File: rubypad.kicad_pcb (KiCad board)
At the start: 2 copper layers, 13 parts, among them U1 ProMicro

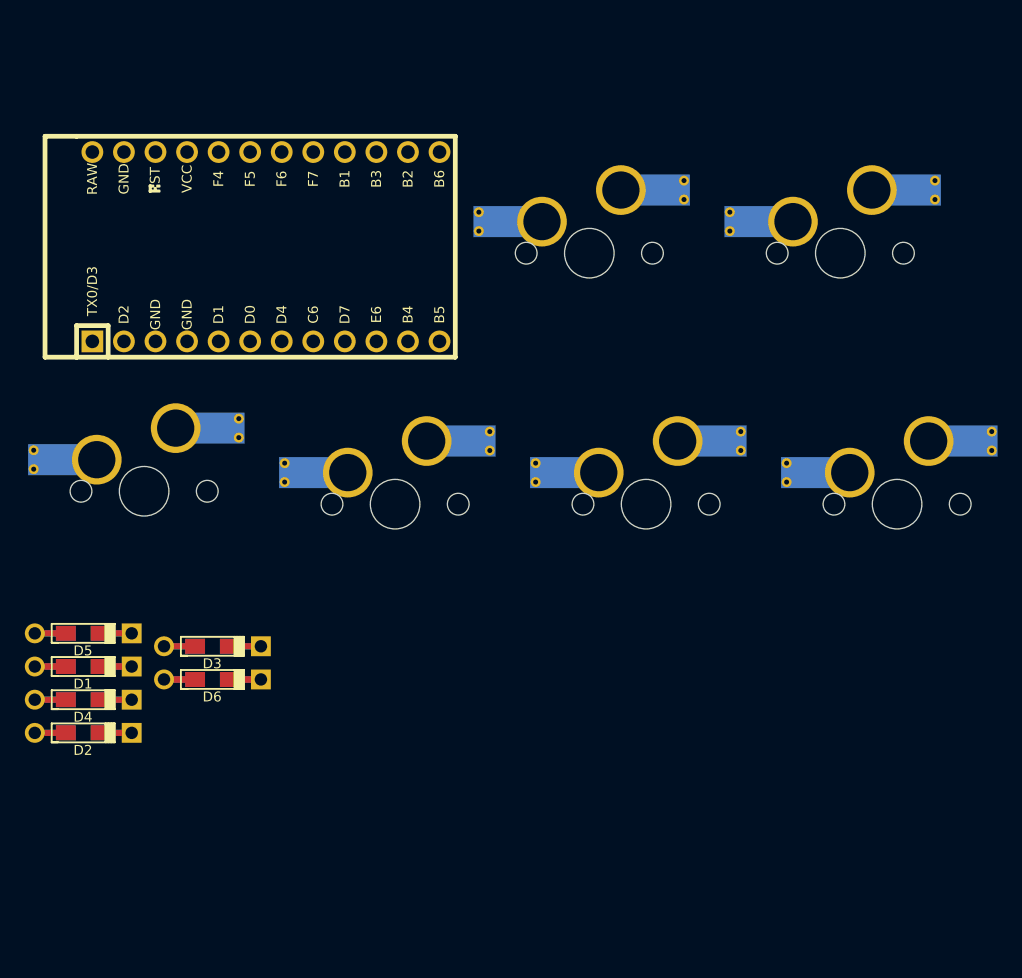
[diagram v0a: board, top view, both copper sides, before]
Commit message: Update - ran traces
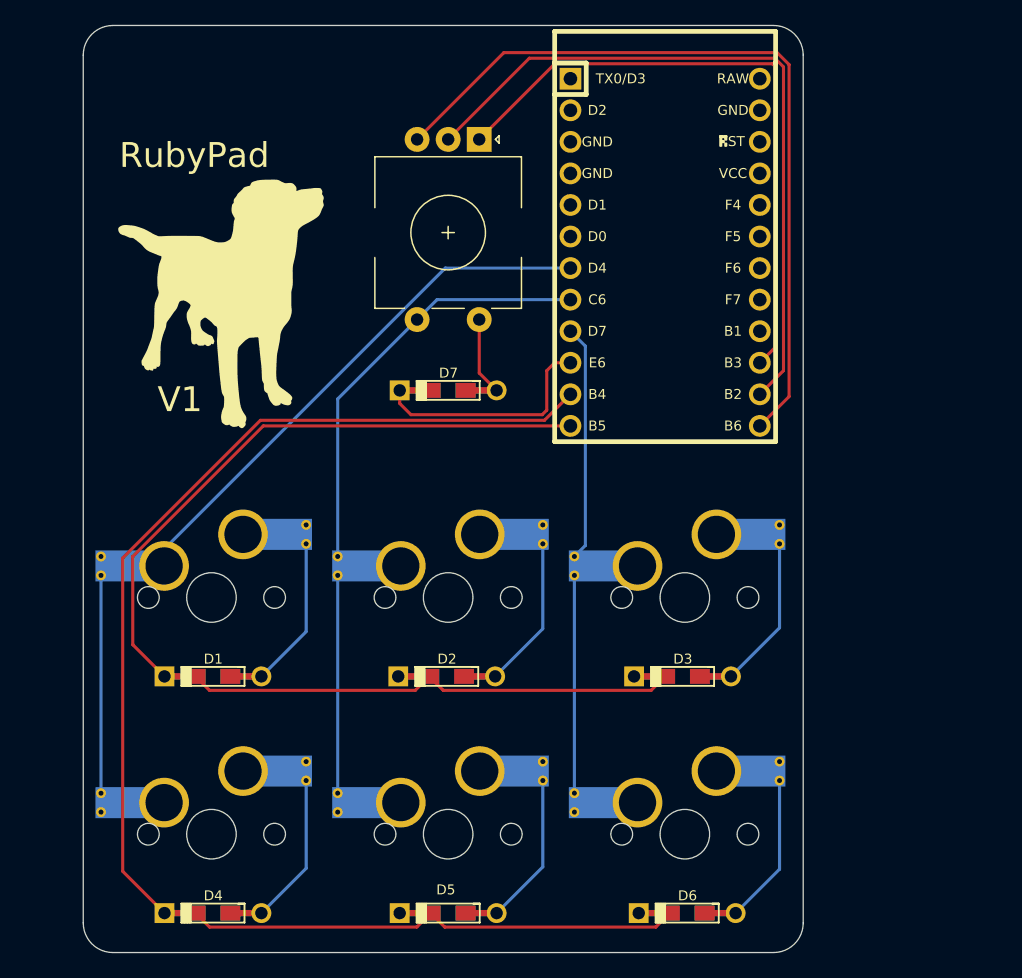
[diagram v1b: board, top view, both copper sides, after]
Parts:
- added D7: D_Small, Keebio-Parts:Diode-dual, F.Cu at (67.5, 47.6)
- added G***: LOGO, rubypad-footprints:logo, F.Cu at (40.9, 27.4)
- added SW1: RotaryEncoder_Switch, Keebio-Parts:RotaryEncoder_EC11, F.Cu at (67.5, 34.9)
- moved MX6 51.5 mm to (86.5, 83.3)
- moved MX4 43.9 mm to (48.4, 83.3)
- moved D6 42.6 mm to (86.7, 89.7), turned to 180 degrees
- moved MX1 41.1 mm to (48.4, 64.3)
- moved D3 37.9 mm to (86.3, 70.6), turned to 180 degrees
- moved D5 37.0 mm to (67.5, 89.7), turned to 180 degrees
- moved MX2 36.9 mm to (67.5, 64.3)
- moved U1 32.1 mm to (84.9, 36.5), turned to -90 degrees
- moved MX3 30.4 mm to (86.5, 64.3)
- moved D2 29.6 mm to (67.3, 70.6), turned to 180 degrees
- moved MX5 26.9 mm to (67.5, 83.3)
- moved D4 20.1 mm to (48.5, 89.7), turned to 180 degrees
- moved D1 10.5 mm to (48.5, 70.6), turned to 180 degrees
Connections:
- D1 pad 1: row0 -> row1
- D2 pad 1: row0 -> row1
- D3 pad 1: row0 -> row1
- D4 pad 1: row1 -> row2
- D5 pad 1: row1 -> row2
- D6 pad 1: row1 -> row2
- U1 pad 10: unconnected-(U1-Pad10) -> row0
- U1 pad 11: unconnected-(U1-Pad11) -> row2
- U1 pad 12: unconnected-(U1-Pad12) -> row1
- U1 pad 13: unconnected-(U1-Pad13) -> ENCB
- U1 pad 14: unconnected-(U1-Pad14) -> ENCC
- U1 pad 15: unconnected-(U1-Pad15) -> ENCA
- U1 pad 7: unconnected-(U1-Pad7) -> col0
- U1 pad 8: unconnected-(U1-Pad8) -> col1
- U1 pad 9: unconnected-(U1-Pad9) -> col2
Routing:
- net row2: track 0.00 -> 111.5 mm
- net row1: track 0.00 -> 89.9 mm
- net ENCB: track 0.00 -> 63.3 mm
- net col0: track 0.00 -> 60.9 mm
- net ENCC: track 0.00 -> 57.1 mm
- net col1: track 0.00 -> 52.2 mm
- net ENCA: track 0.00 -> 50.8 mm
- net col2: track 0.00 -> 36.5 mm
- net row0: track 0.00 -> 18.8 mm
- net Net-(D3-Pad2): track 0.00 -> 12.3 mm
- net Net-(D2-Pad2): track 0.00 -> 12.3 mm
- net Net-(D5-Pad2): track 0.00 -> 12.2 mm
- net Net-(D1-Pad2): track 0.00 -> 12.2 mm
- net Net-(D4-Pad2): track 0.00 -> 12.2 mm
- net Net-(D6-Pad2): track 0.00 -> 12.1 mm
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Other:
- board outline added: 57.9 x 74.6 mm
